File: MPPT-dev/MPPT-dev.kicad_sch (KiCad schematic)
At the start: 3 parts, among them J1 200528-0100, J13 282834-6, J2 Conn_01x02

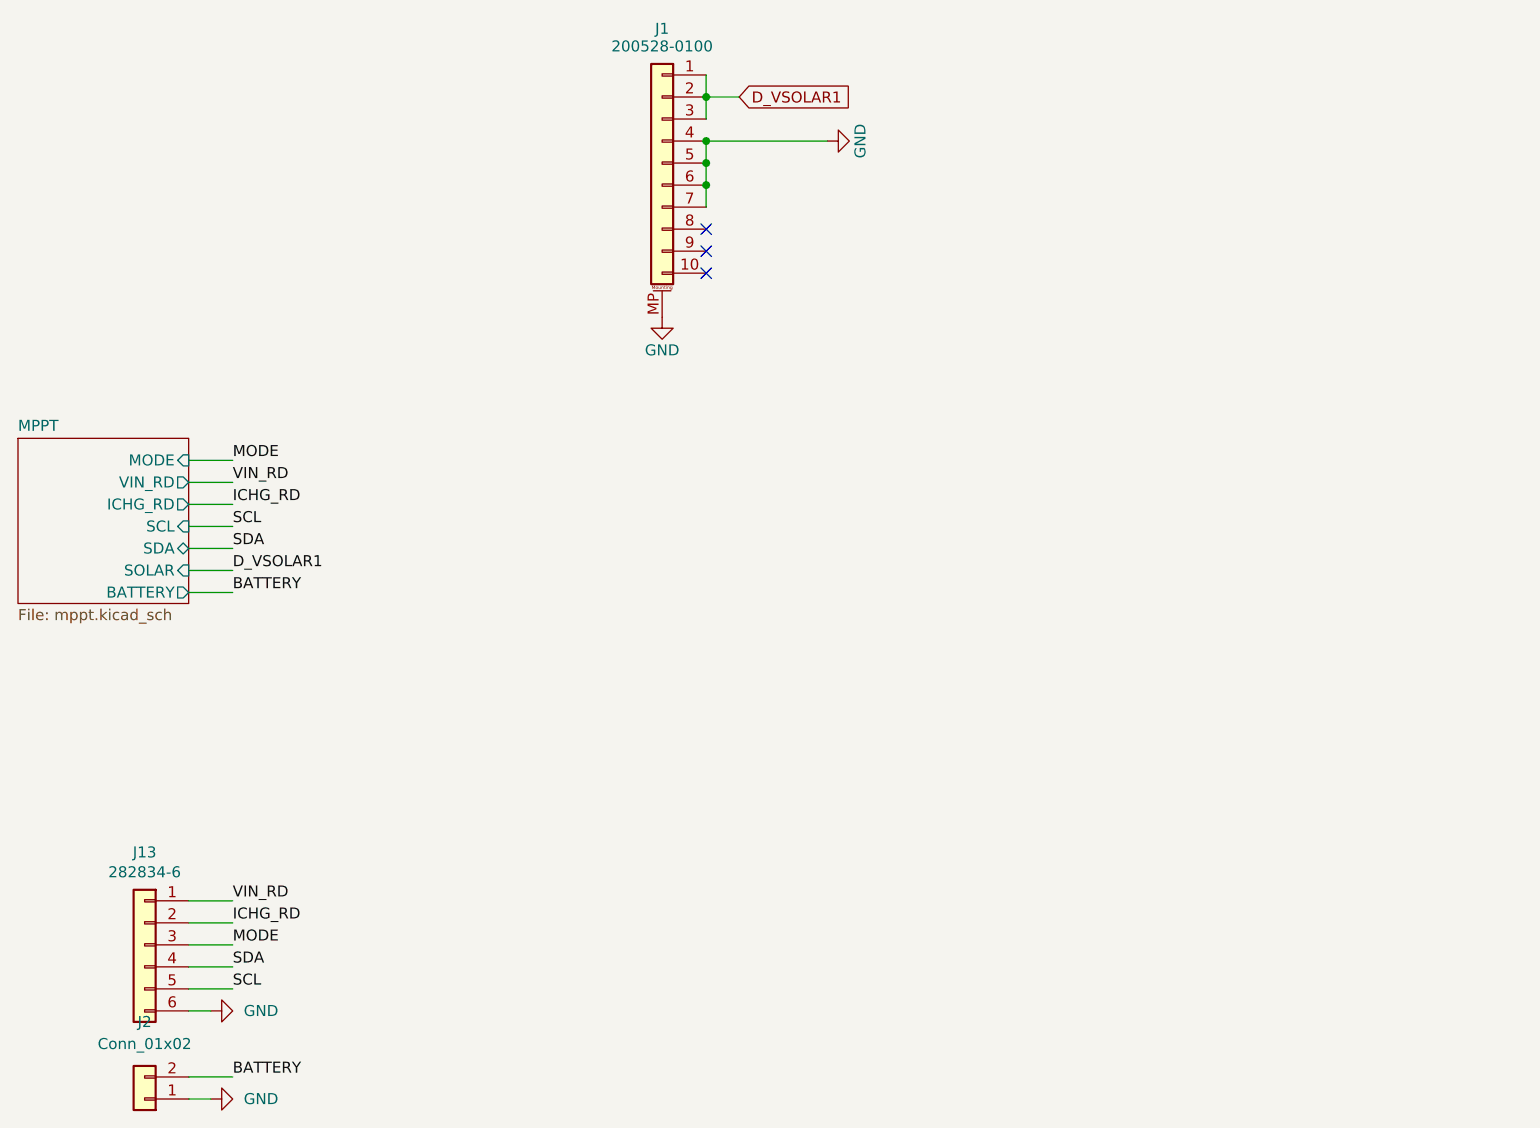
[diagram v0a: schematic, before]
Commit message: Board review
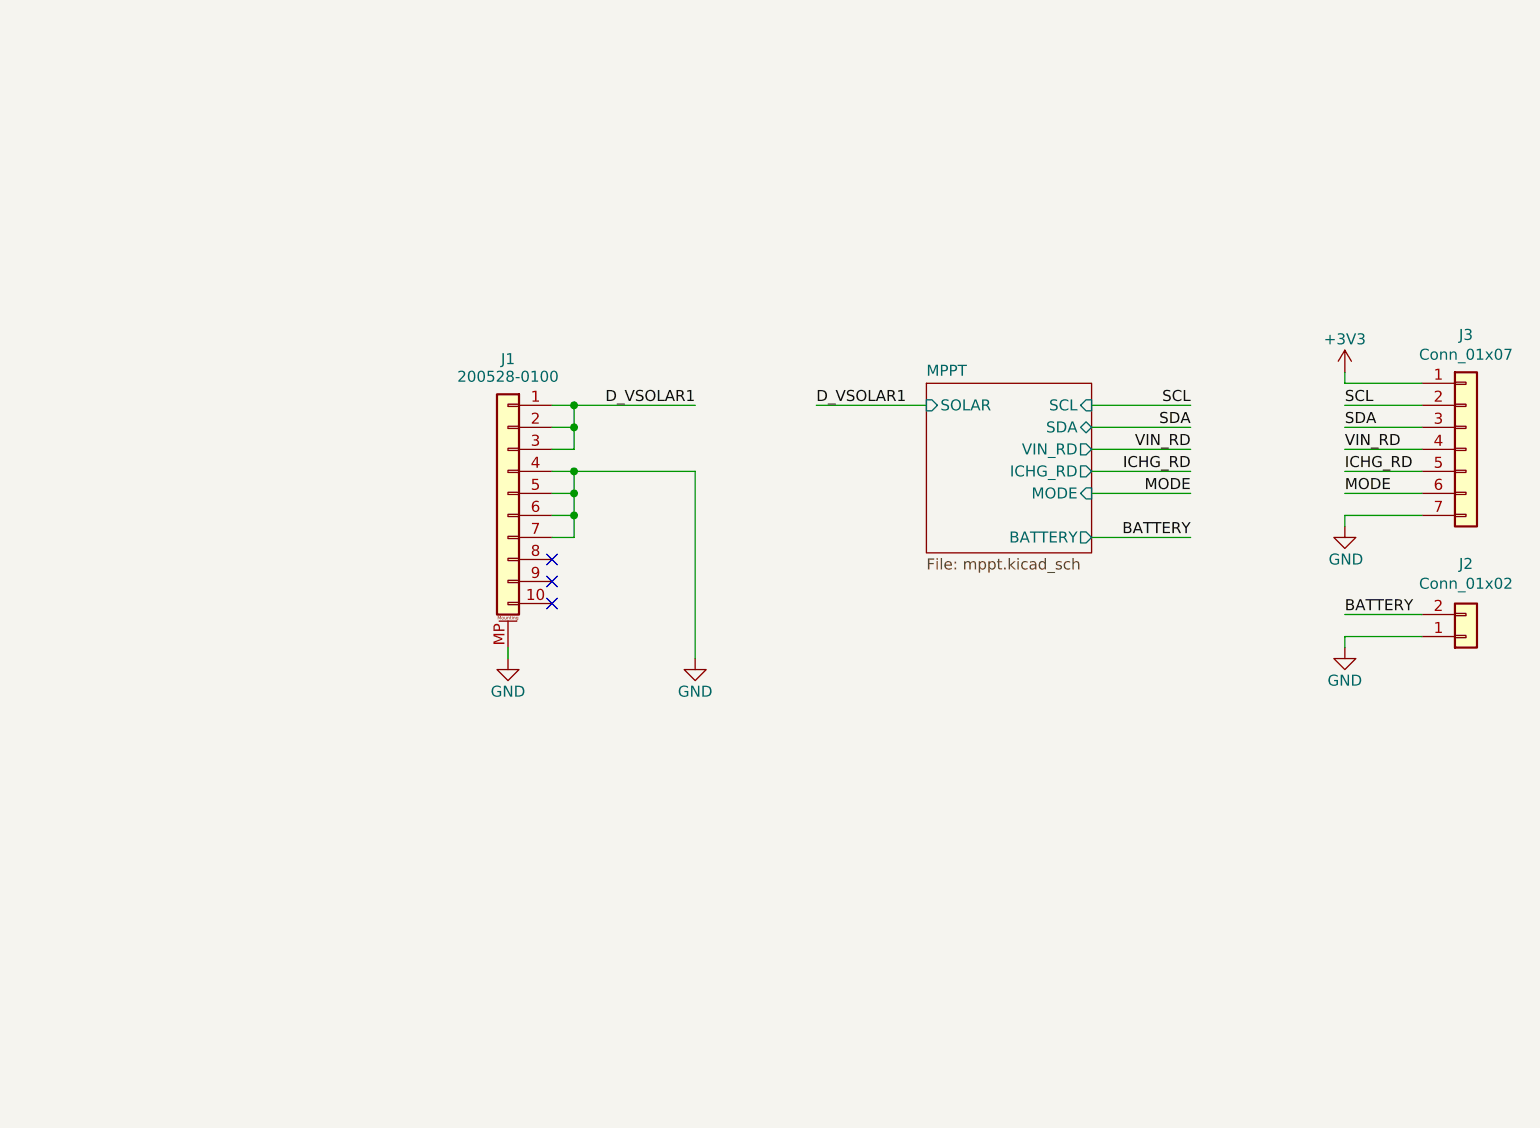
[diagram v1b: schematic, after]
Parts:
- J1: footprint Argus-Connectors:Molex_200528-0100_1x10-1MP_P1.00mm_Horizontal -> footprints:Molex_200528-0100_1x10-1MP_P1.00mm_Horizontal
- J3: renamed from J13; value 282834-6 -> Conn_01x07; footprint Connector_PinHeader_2.54mm:PinHeader_1x06_P2.54mm_Vertical -> Connector_PinHeader_2.54mm:PinHeader_1x07_P2.54mm_Vertical; symbol Connector_Generic:Conn_01x06 -> Connector_Generic:Conn_01x07
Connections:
- net GND: now also J3.7 (Pin_7); no longer J3.6 (Pin_6)
- net ICHG_RD: now also J3.5 (Pin_5); no longer J3.2 (Pin_2)
- net MODE: now also J3.6 (Pin_6); no longer J3.3 (Pin_3)
- net SCL: now also J3.2 (Pin_2); no longer J3.5 (Pin_5)
- net SDA: now also J3.3 (Pin_3); no longer J3.4 (Pin_4)
- net VIN_RD: now also J3.4 (Pin_4); no longer J3.1 (Pin_1)
- new net +3V3: J3.1 (Pin_1)
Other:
- moved on the sheet: J1, J2
